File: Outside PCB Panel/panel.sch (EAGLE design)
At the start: 1 part, among them J2 641737-1

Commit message: did PCB panel
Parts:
- added IC1, IC2, IC3, IC4, IC5, IC6, IC7, IC8: LD117AS12TR, v-reg:LD117AS12TR
- added U$1, U$10, U$11, U$12, U$13, U$14, U$15, U$16, U$17, U$18, U$19, U$2, U$20, U$21, U$22, U$23, U$24, U$25, U$26, U$27, U$28, U$29, U$3, U$30, U$31, U$32, U$33, U$34, U$35, U$36, U$37, U$38, U$39, U$4, U$40, U$41, U$42, U$43, U$44, U$45, U$46, U$47, U$48, U$49, U$5, U$50, U$51, U$52, U$53, U$54, U$55, U$56, U$57, U$58, U$59, U$6, U$60, U$61, U$62, U$63, U$64, U$65, U$66, U$67, U$68, U$69, U$7, U$70, U$71, U$72, U$73, U$74, U$75, U$76, U$77, U$78, U$79, U$8, U$80, U$81, U$82, U$83, U$84, U$85, U$9: SAO1.69BIS, ShittyAddOn:SAO1.69BIS
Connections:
- new net 3V3: IC1.OUT, IC2.OUT, IC3.OUT, IC4.OUT, IC5.OUT, IC6.OUT, IC7.OUT, IC8.OUT, U$1.3V3, U$10.3V3, U$11.3V3, U$12.3V3, U$13.3V3, U$14.3V3, U$15.3V3, U$16.3V3, U$17.3V3, U$18.3V3, U$19.3V3, U$2.3V3, U$20.3V3, U$21.3V3, U$22.3V3, U$23.3V3, U$24.3V3, U$25.3V3, U$26.3V3, U$27.3V3, U$28.3V3, U$29.3V3, U$3.3V3, U$30.3V3, U$31.3V3, U$32.3V3, U$33.3V3, U$34.3V3, U$35.3V3, U$36.3V3, U$37.3V3, U$38.3V3, U$39.3V3, U$4.3V3, U$40.3V3, U$41.3V3, U$42.3V3, U$43.3V3, U$44.3V3, U$45.3V3, U$46.3V3, U$47.3V3, U$48.3V3, U$49.3V3, U$5.3V3, U$50.3V3, U$51.3V3, U$52.3V3, U$53.3V3, U$54.3V3, U$55.3V3, U$56.3V3, U$57.3V3, U$58.3V3, U$59.3V3, U$6.3V3, U$60.3V3, U$61.3V3, U$62.3V3, U$63.3V3, U$64.3V3, U$65.3V3, U$66.3V3, U$67.3V3, U$68.3V3, U$69.3V3, U$7.3V3, U$70.3V3, U$71.3V3, U$72.3V3, U$73.3V3, U$74.3V3, U$75.3V3, U$76.3V3, U$77.3V3, U$78.3V3, U$79.3V3, U$8.3V3, U$80.3V3, U$81.3V3, U$82.3V3, U$83.3V3, U$84.3V3, U$85.3V3, U$9.3V3
- net 5V: now also IC1.IN, IC2.IN, IC3.IN, IC4.IN, IC5.IN, IC6.IN, IC7.IN, IC8.IN
- net GND: now also IC1.ADJ, IC2.ADJ, IC3.ADJ, IC4.ADJ, IC5.ADJ, IC6.ADJ, IC7.ADJ, IC8.ADJ, U$1.GND, U$10.GND, U$11.GND, U$12.GND, U$13.GND, U$14.GND, U$15.GND, U$16.GND, U$17.GND, U$18.GND, U$19.GND, U$2.GND, U$20.GND, U$21.GND, U$22.GND, U$23.GND, U$24.GND, U$25.GND, U$26.GND, U$27.GND, U$28.GND, U$29.GND, U$3.GND, U$30.GND, U$31.GND, U$32.GND, U$33.GND, U$34.GND, U$35.GND, U$36.GND, U$37.GND, U$38.GND, U$39.GND, U$4.GND, U$40.GND, U$41.GND, U$42.GND, U$43.GND, U$44.GND, U$45.GND, U$46.GND, U$47.GND, U$48.GND, U$49.GND, U$5.GND, U$50.GND, U$51.GND, U$52.GND, U$53.GND, U$54.GND, U$55.GND, U$56.GND, U$57.GND, U$58.GND, U$59.GND, U$6.GND, U$60.GND, U$61.GND, U$62.GND, U$63.GND, U$64.GND, U$65.GND, U$66.GND, U$67.GND, U$68.GND, U$69.GND, U$7.GND, U$70.GND, U$71.GND, U$72.GND, U$73.GND, U$74.GND, U$75.GND, U$76.GND, U$77.GND, U$78.GND, U$79.GND, U$8.GND, U$80.GND, U$81.GND, U$82.GND, U$83.GND, U$84.GND, U$85.GND, U$9.GND

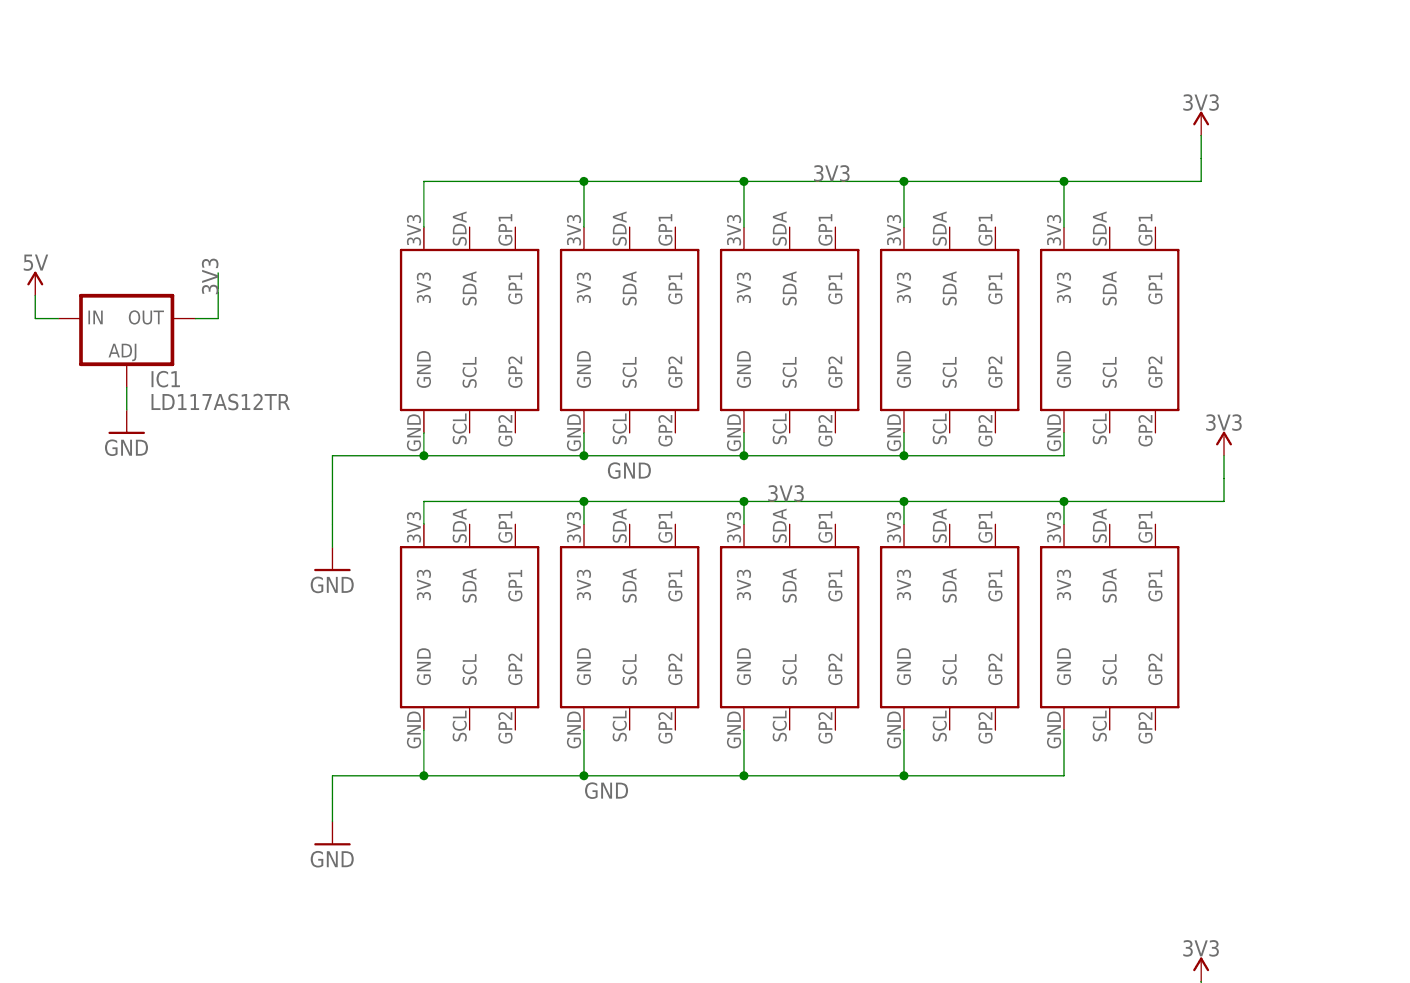
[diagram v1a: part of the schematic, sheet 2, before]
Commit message: Fixed panel
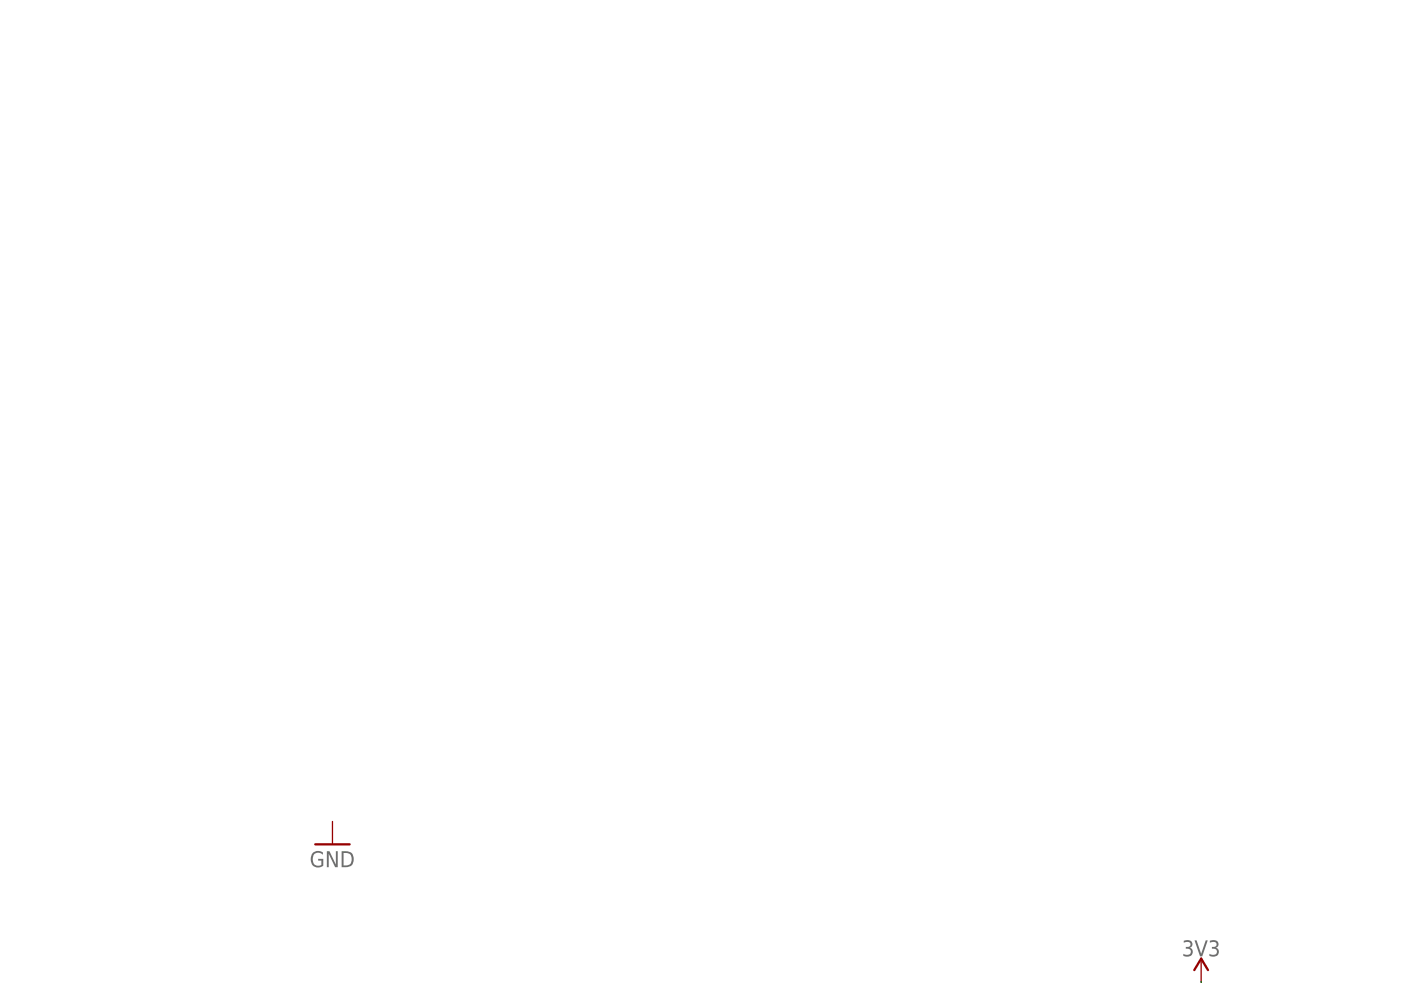
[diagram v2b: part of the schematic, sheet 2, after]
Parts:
- removed IC1: LD117AS12TR, v-reg:LD117AS12TR
- removed U$1, U$10, U$2, U$3, U$4, U$5, U$6, U$7, U$8, U$9: SAO1.69BIS, ShittyAddOn:SAO1.69BIS
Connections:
- net 3V3: no longer IC1.OUT, U$1.3V3, U$10.3V3, U$2.3V3, U$3.3V3, U$4.3V3, U$5.3V3, U$6.3V3, U$7.3V3, U$8.3V3, U$9.3V3
- net 5V: no longer IC1.IN
- net GND: no longer IC1.ADJ, U$1.GND, U$10.GND, U$2.GND, U$3.GND, U$4.GND, U$5.GND, U$6.GND, U$7.GND, U$8.GND, U$9.GND
